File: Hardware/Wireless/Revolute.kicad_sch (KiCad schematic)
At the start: 52 parts, among them U1 BQ27441-G1, U2 Button, U2 nrf52833_qfn40, U3 AS5600, U4 AP2112K-3.3, U5 BQ24075RGT, X1 32.768 kHz, X2 32MHZ

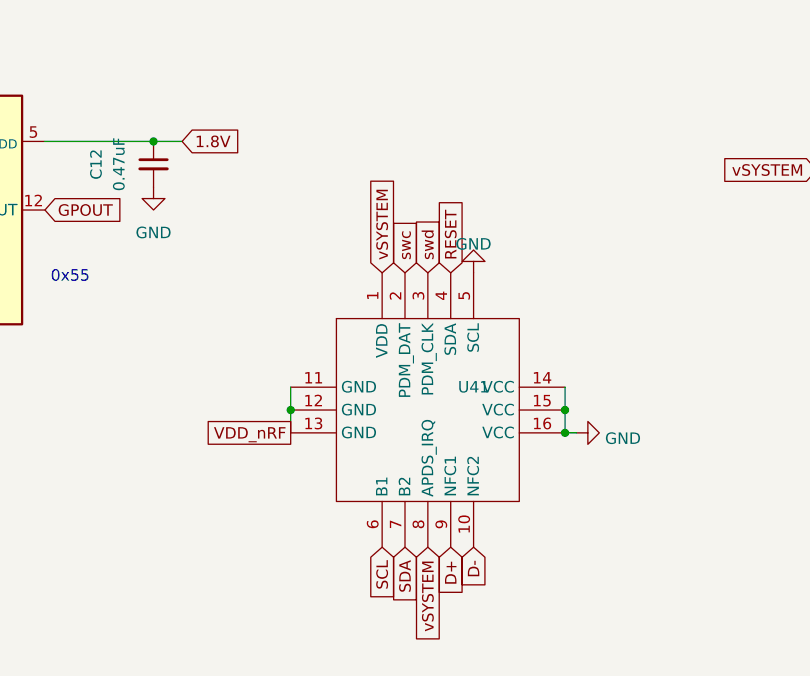
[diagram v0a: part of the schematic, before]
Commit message: fixed design
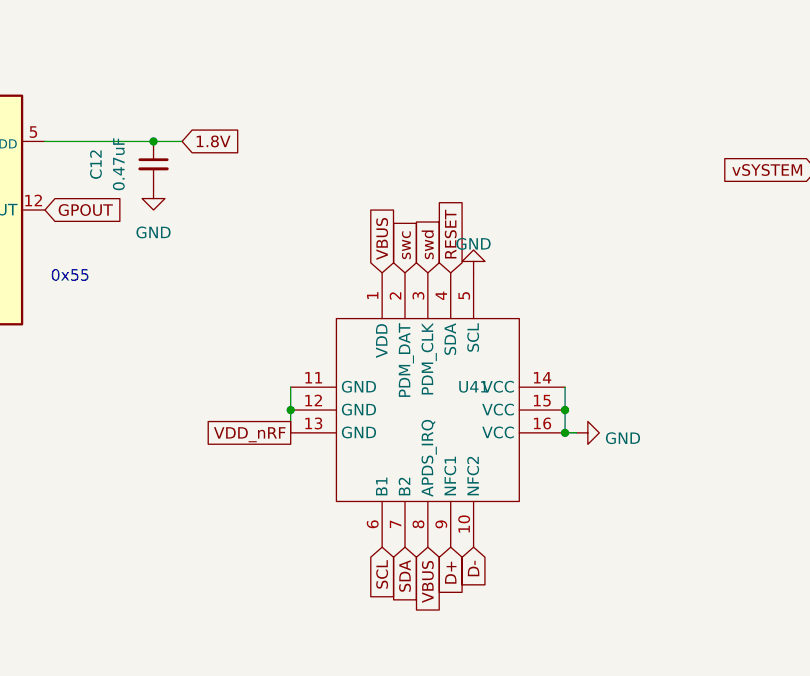
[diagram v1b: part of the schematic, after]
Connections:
- net OUT: no longer U41.1 (VDD), U41.8 (APDS_IRQ)
- net VBUS: now also U41.1 (VDD), U41.8 (APDS_IRQ)
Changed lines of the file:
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@@
-    )
-  )
-  (global_label "vSYSTEM" (shape input) (at 115.57 151.765 90) (fields_autoplaced)
-    (effects (font (size 1.27 1.27)) (justify left))
-    (property "Intersheetrefs" "${INTERSHEET_REFS}" (at 115.57 140.816 90)
-      (effects (font (size 1.27 1.27)) (justify left) hide)
     )
   )
@@
     )
   )
+  (global_label "VBUS" (shape input) (at 115.57 151.765 90) (fields_autoplaced)
+    (effects (font (size 1.27 1.27)) (justify left))
+    (property "Intersheetrefs" "${INTERSHEET_REFS}" (at 115.57 143.9606 90)
+      (effects (font (size 1.27 1.27)) (justify left) hide)
+    )
+  )
   (global_label "swc" (shape input) (at 118.11 151.765 90) (fields_autoplaced)
     (effects (font (size 1.27 1.27)) (justify left))
@@
     )
   )
+  (global_label "VBUS" (shape input) (at 120.65 182.245 270) (fields_autoplaced)
+    (effects (font (size 1.27 1.27)) (justify right))
+    (property "Intersheetrefs" "${INTERSHEET_REFS}" (at 120.65 190.0494 90)
+      (effects (font (size 1.27 1.27)) (justify right) hide)
+    )
+  )
   (global_label "OUT" (shape input) (at 211.455 37.465 270) (fields_autoplaced)
     (effects (font (size 1.27 1.27)) (justify right))
@@
     )
   )
-  (global_label "vSYSTEM" (shape input) (at 120.65 182.245 270) (fields_autoplaced)
-    (effects (font (size 1.27 1.27)) (justify right))
-    (property "Intersheetrefs" "${INTERSHEET_REFS}" (at 120.65 193.194 90)
-      (effects (font (size 1.27 1.27)) (justify right) hide)
-    )
-  )
